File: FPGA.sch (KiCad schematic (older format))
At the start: 0 parts

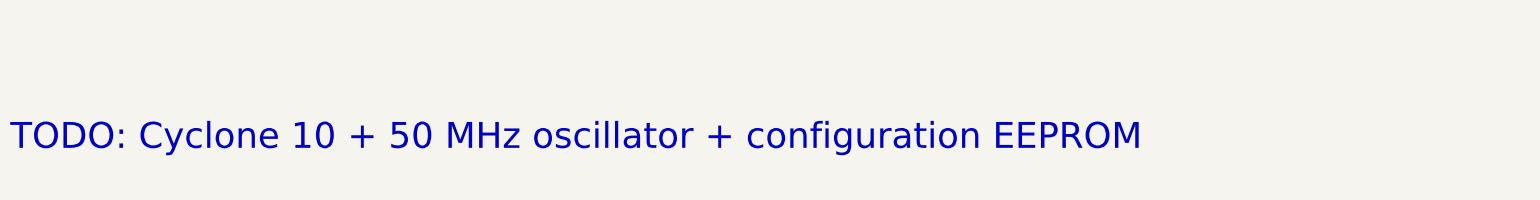
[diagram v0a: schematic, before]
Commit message: Add TODO notes
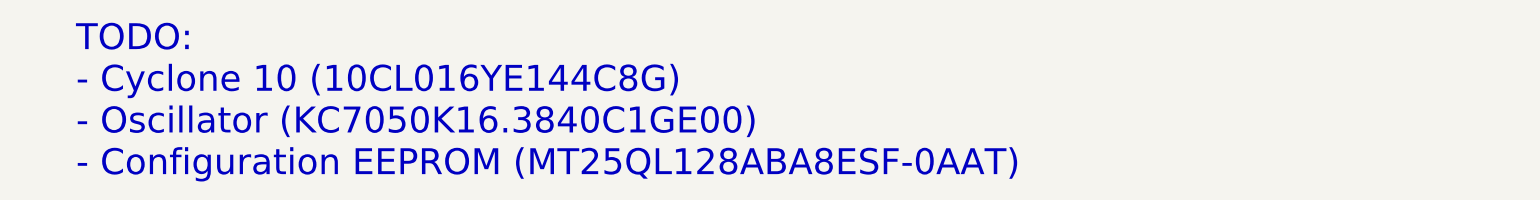
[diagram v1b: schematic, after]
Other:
- note added: "TODO:\n- Cyclone 10 (10CL016YE144C8G)\n- Oscillator (KC7050K16.3840C1GE00)\n- Configuration EEPROM (MT25QL128ABA8ESF-0AAT)"
- note removed: "TODO: Cyclone 10 + 50 MHz oscillator + configuration EEPROM"
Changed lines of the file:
@@
 Comment4 ""
 $EndDescr
-Text Notes 1000 3950 0    197  ~ 0
-TODO: Cyclone 10 + 50 MHz oscillator + configuration EEPROM
+Text Notes 1500 4150 0    197  ~ 0
+TODO:\n- Cyclone 10 (10CL016YE144C8G)\n- Oscillator (KC7050K16.3840C1GE00)\n- Configuration EEPROM (MT25QL128ABA8ESF-0AAT)
 $EndSCHEMATC
